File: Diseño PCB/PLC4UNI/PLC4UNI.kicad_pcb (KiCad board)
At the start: 2 copper layers, 2 parts, among them J2 Screw_Terminal_01x18

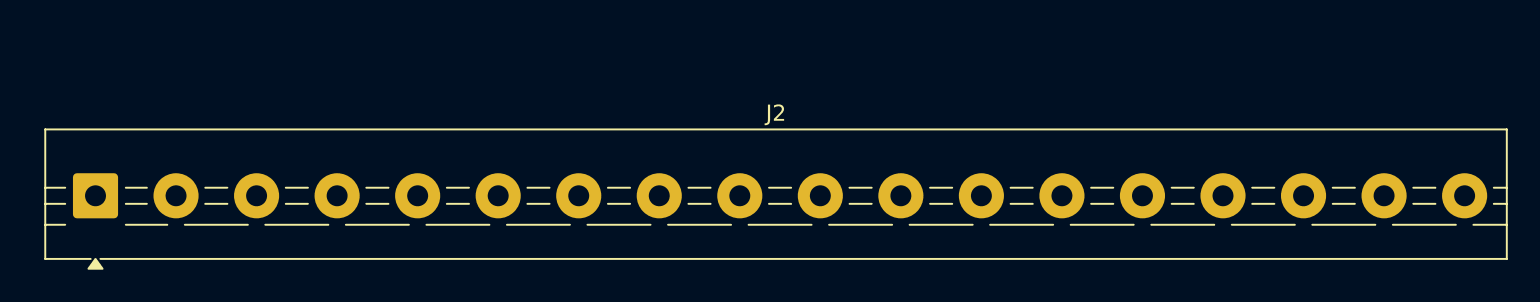
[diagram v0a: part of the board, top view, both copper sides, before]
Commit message: Diseño PCB KiCad
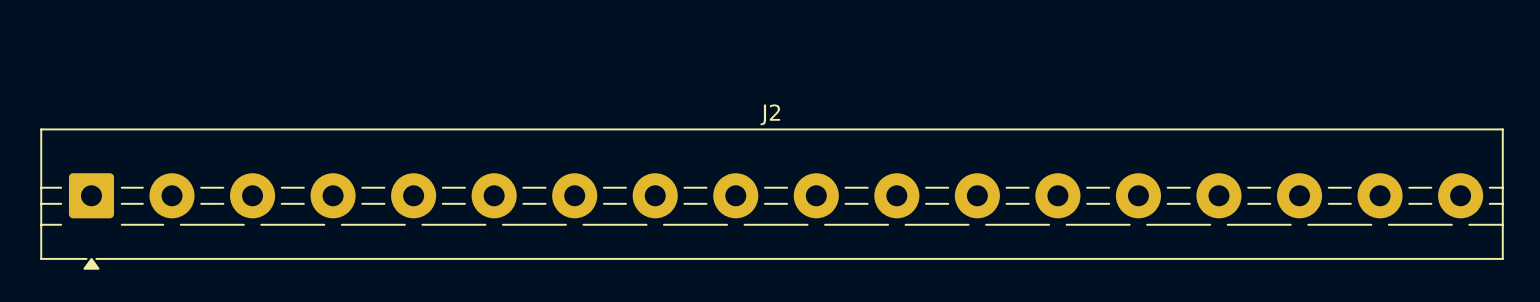
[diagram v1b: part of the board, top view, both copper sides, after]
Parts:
- moved J2 0.25 mm to (70.5, 113.0)
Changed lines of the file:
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@@
 	(footprint "TerminalBlock:TerminalBlock_MaiXu_MX126-5.0-18P_1x18_P5.00mm"
 		(layer "F.Cu")
-		(at 70.75 112.9675)
+		(at 70.5 112.9675)
 		(descr "terminal block MaiXu MX126-5.0-18P, 18 pins, pitch 5mm, size 90.5x7.8mm, drill diameter 1.3mm, pad diameter 2.8mm, https://www.lcsc.com/datasheet/lcsc_datasheet_2309150913_MAX-MX126-5-0-03P-GN01-Cu-S-A_C5188435.pdf, script-generated using https://gitlab.com/kicad/libraries/kicad-footprint-generator/-/tree/master/scripts/TerminalBlock_MaiXu")
 		(tags "THT terminal block MaiXu MX126-5.0-18P pitch 5mm size 90.5x7.8mm drill 1.3mm pad 2.8mm")
